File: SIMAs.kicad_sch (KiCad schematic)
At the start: 10 parts, among them J10 Conn_01x02_Pin, J3 Conn_01x04_Socket, J4 Conn_01x04_Socket, J5 Conn_01x04_Socket, J6 Conn_01x03_Socket, J9 Conn_01x03_Socket, U1 mini_esp32

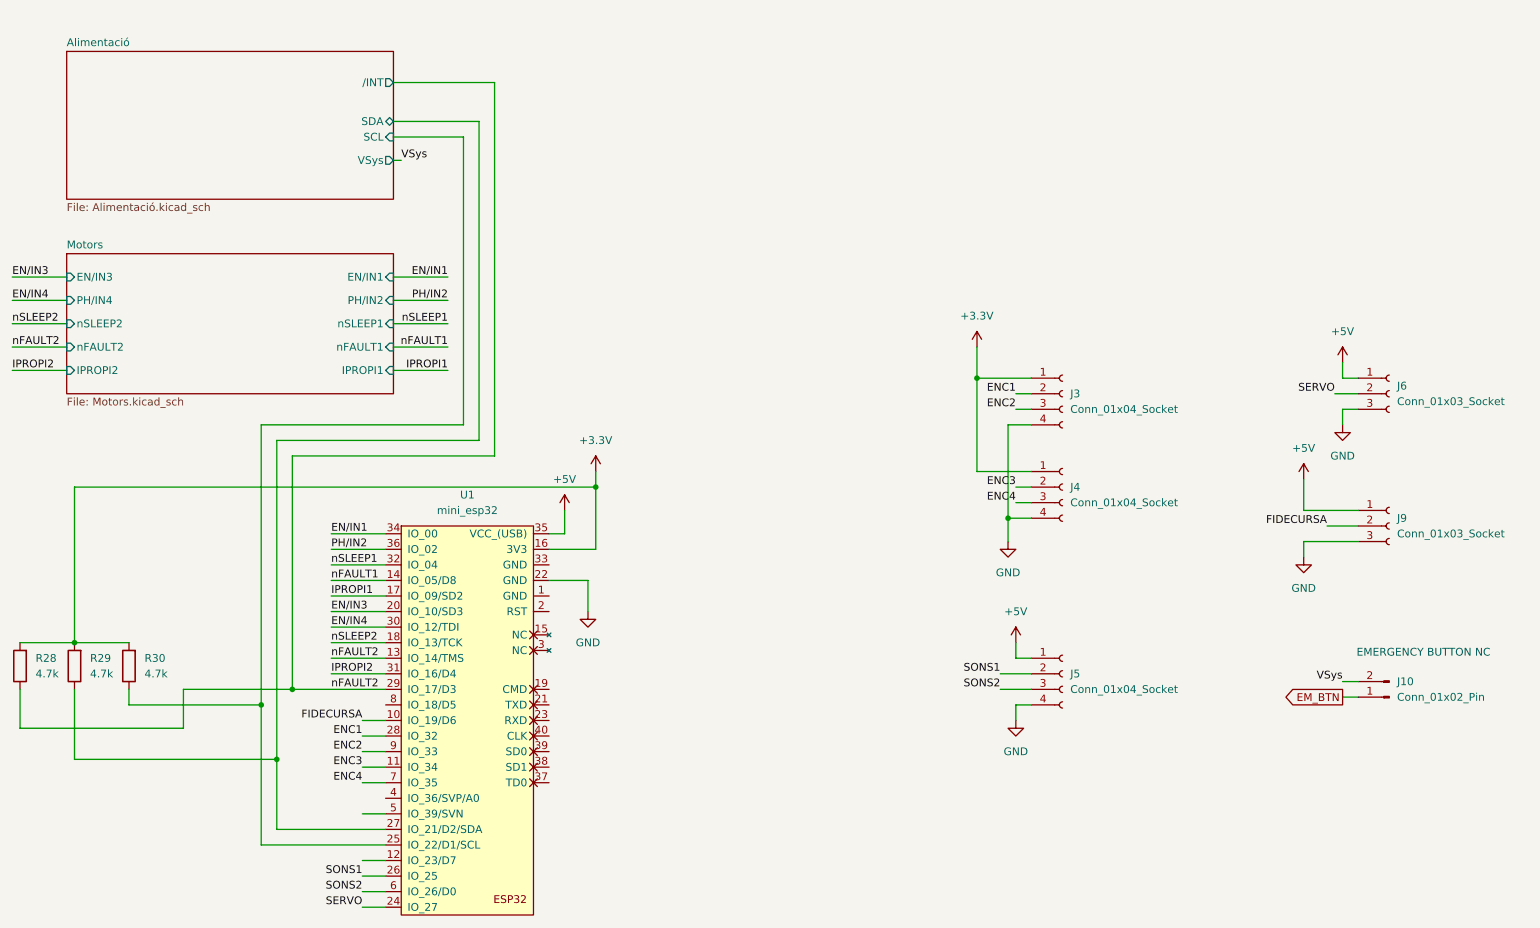
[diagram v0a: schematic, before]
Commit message: Revisio de la placa
S'ha revisat la placa
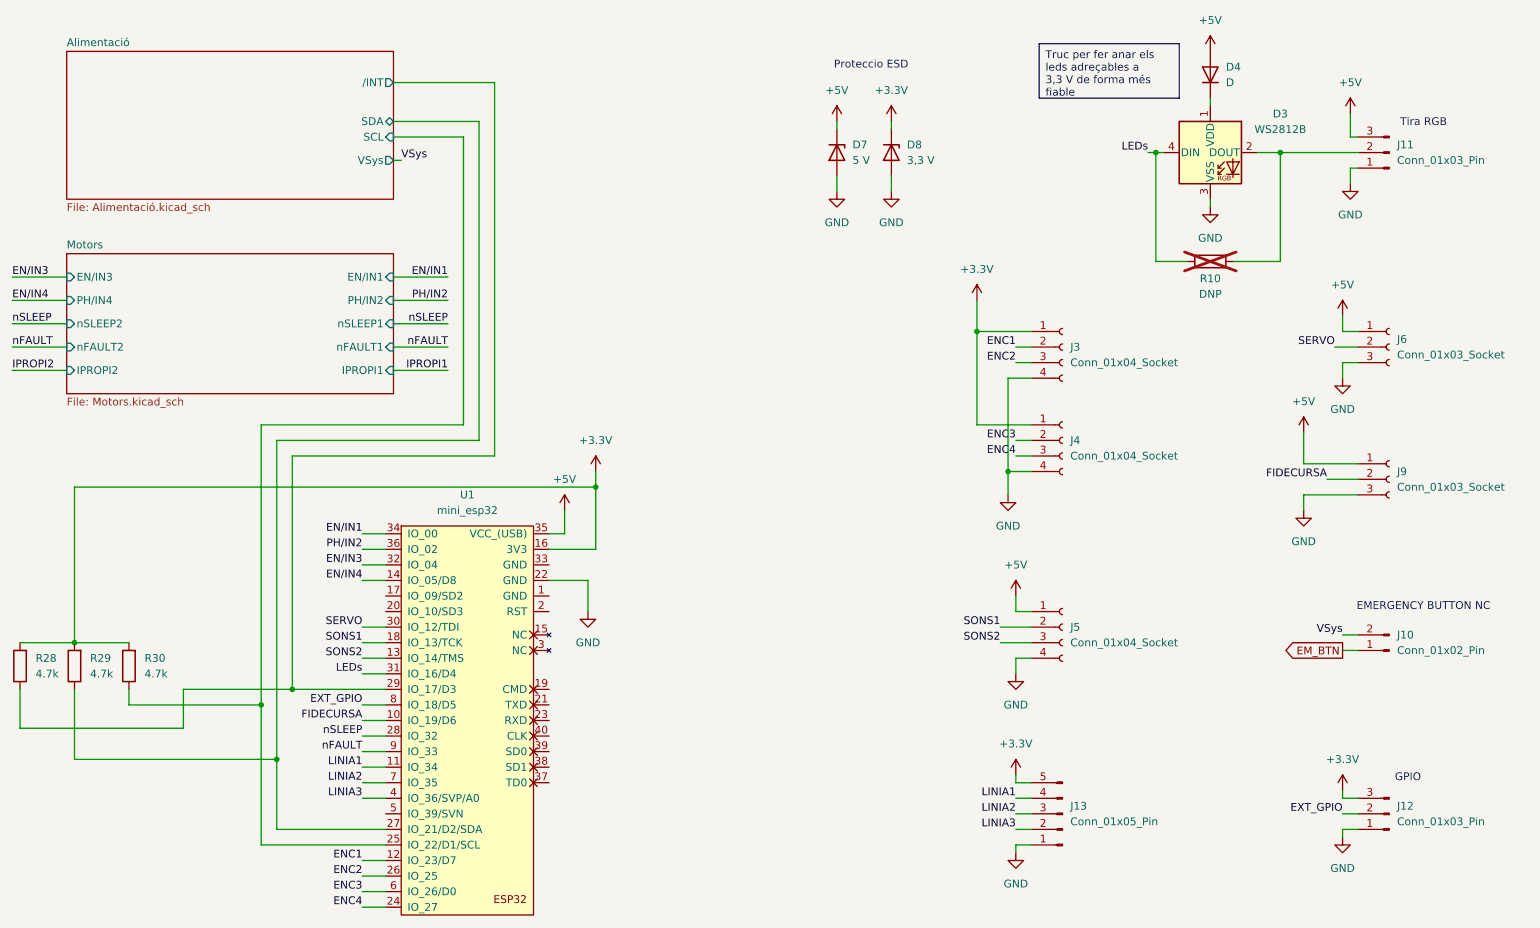
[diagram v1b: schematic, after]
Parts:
- added D3: WS2812B, LED_SMD:LED_WS2812B_PLCC4_5.0x5.0mm_P3.2mm, symbol LED:WS2812B
- added D4: D, Diode_SMD:D_SMA_Handsoldering, symbol Device:D
- added D7: 5 V, Diode_SMD:D_SOD-323, symbol Device:D_Zener
- added D8: 3,3 V, Diode_SMD:D_SOD-323, symbol Device:D_Zener
- added J11, J12: Conn_01x03_Pin, Connector_JST:JST_PH_B3B-PH-K_1x03_P2.00mm_Vertical, symbol Connector:Conn_01x03_Pin
- added J13: Conn_01x05_Pin, Connector_JST:JST_PH_B5B-PH-K_1x05_P2.00mm_Vertical, symbol Connector:Conn_01x05_Pin
- added R10: DNP, Resistor_SMD:R_0603_1608Metric, symbol Device:R
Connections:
- net nFAULT1 is gone; now on net EN/IN4: U1.14 (IO_05/D8)
- net nSLEEP1 is gone; now on net EN/IN3: U1.32 (IO_04)
- net nSLEEP2 is gone; now on net SONS1: U1.18 (IO_13/TCK)
- net +3.3V: now also D8.1 (K), J12.3 (Pin_3), J13.5 (Pin_5)
- net +5V: now also D4.2 (A), D7.1 (K), J11.3 (Pin_3)
- net ENC1: now also U1.12 (IO_23/D7); no longer U1.28 (IO_32)
- net ENC2: now also U1.26 (IO_25); no longer U1.9 (IO_33)
- net ENC3: now also U1.6 (IO_26/D0); no longer U1.11 (IO_34)
- net ENC4: now also U1.24 (IO_27); no longer U1.7 (IO_35)
- net EN/IN3: no longer U1.20 (IO_10/SD3)
- net EN/IN4: no longer U1.30 (IO_12/TDI)
- net GND: now also D3.3 (VSS), D7.2 (A), D8.2 (A), J11.1 (Pin_1), J12.1 (Pin_1), J13.1 (Pin_1)
- net IPROPI1: no longer U1.17 (IO_09/SD2)
- net IPROPI2: no longer U1.31 (IO_16/D4)
- net SERVO: now also U1.30 (IO_12/TDI); no longer U1.24 (IO_27)
- net SONS1: no longer U1.26 (IO_25)
- net SONS2: now also U1.13 (IO_14/TMS); no longer U1.6 (IO_26/D0)
- net LINIA3: now reaches U1.4 (IO_36/SVP/A0)
- net LINIA3: now also J13.2 (Pin_2)
- net EXT_GPIO: now reaches U1.8 (IO_18/D5)
- net EXT_GPIO: now also J12.2 (Pin_2)
- net nFAULT2 renamed Alimentació//INT
- net Alimentació//INT: no longer U1.13 (IO_14/TMS)
- new net: D3.2 (DOUT), J11.2 (Pin_2), R10.2
- new net: D3.1 (VDD), D4.1 (K)
- new net LEDs: D3.4 (DIN), R10.1, U1.31 (IO_16/D4)
- new net LINIA1: J13.4 (Pin_4), U1.11 (IO_34)
- new net LINIA2: J13.3 (Pin_3), U1.7 (IO_35)
- new net nFAULT: U1.9 (IO_33)
- new net nSLEEP: U1.28 (IO_32)
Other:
- note added: "GPIO"
- note added: "Proteccio ESD"
- note added: "Tira RGB"
- moved on the sheet: J10, J3, J4, J5, J6, J9
